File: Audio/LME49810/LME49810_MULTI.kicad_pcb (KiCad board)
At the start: 2 copper layers, 165.1 x 190.5 mm, 124 parts, among them Q1 NPN(TO-3P-BCE), Q2 PNP(TO-3P-BCE), Q3 NPN(TO-220-BCE), U1 LME49810

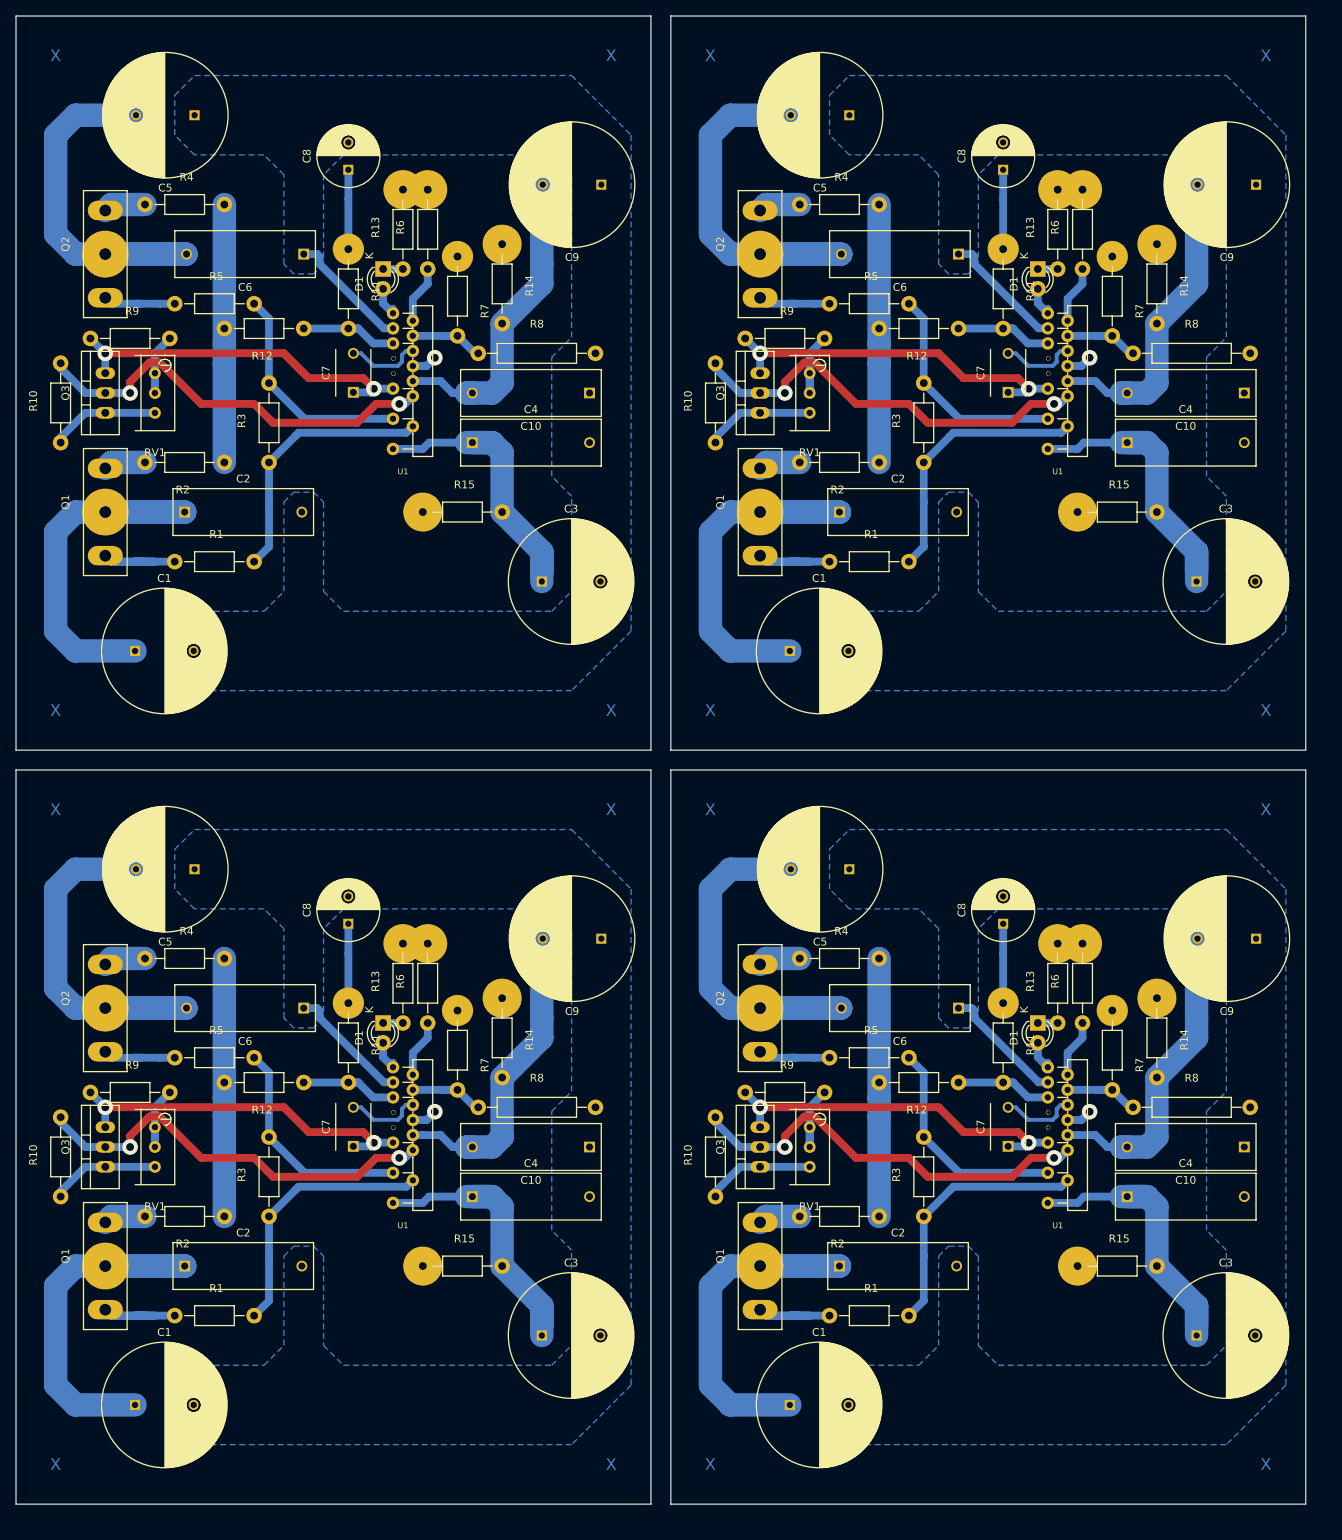
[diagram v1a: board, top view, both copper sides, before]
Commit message: Fixes
More fixes done
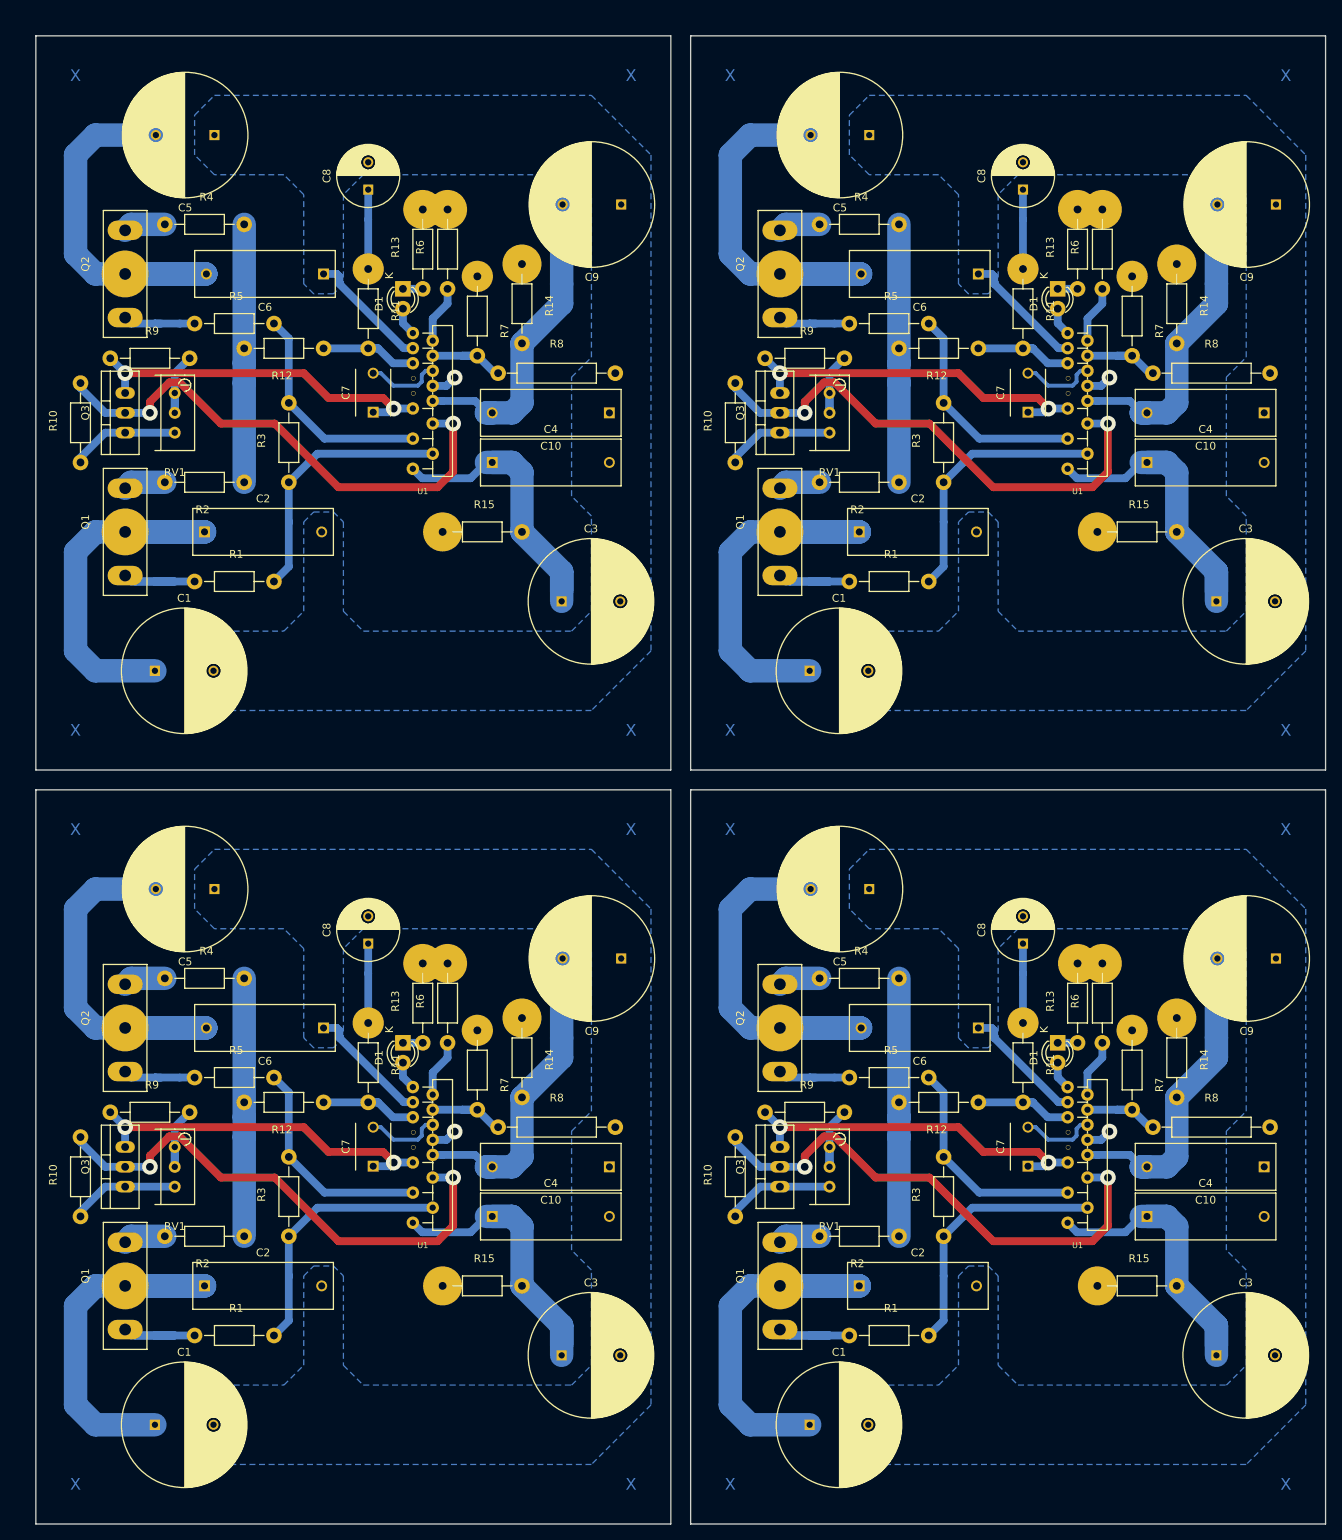
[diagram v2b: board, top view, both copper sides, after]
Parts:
- removed the C1 at (33.0, 99.1)
- removed the C1 at (116.8, 99.1)
- removed the C1 at (33.0, 195.6)
- removed the C1 at (116.8, 195.6)
- removed the C10 at (91.2, 66.0)
- removed the C10 at (175.0, 66.0)
- removed the C10 at (91.2, 162.6)
- removed the C10 at (175.0, 162.6)
- removed the C2 at (39.4, 81.3)
- removed the C2 at (123.2, 81.3)
- removed the C2 at (39.4, 177.8)
- removed the C2 at (123.2, 177.8)
- removed the C3 at (85.1, 90.2)
- removed the C3 at (168.9, 90.2)
- removed the C3 at (85.1, 186.7)
- removed the C3 at (168.9, 186.7)
- removed the C4 at (76.2, 72.4)
- removed the C4 at (160.0, 72.4)
- removed the C4 at (76.2, 168.9)
- removed the C4 at (160.0, 168.9)
- removed the C5 at (40.6, 30.5)
- removed the C5 at (124.5, 30.5)
- removed the C5 at (40.6, 127.0)
- removed the C5 at (124.5, 127.0)
- removed the C6 at (54.6, 48.3)
- removed the C6 at (138.4, 48.3)
- removed the C6 at (54.6, 144.8)
- removed the C6 at (138.4, 144.8)
- removed the C7 at (61.0, 66.0)
- removed the C7 at (144.8, 66.0)
- removed the C7 at (61.0, 162.5)
- removed the C7 at (144.8, 162.5)
- removed the C8 at (60.3, 37.5)
- removed the C8 at (144.1, 37.5)
- removed the C8 at (60.3, 134.0)
- removed the C8 at (144.1, 134.0)
- removed the C9 at (92.7, 39.4)
- removed the C9 at (176.5, 39.4)
- removed the C9 at (92.7, 135.9)
- removed the C9 at (176.5, 135.9)
- removed the D1 at (64.8, 50.2)
- removed the D1 at (148.6, 50.2)
- removed the D1 at (64.8, 146.7)
- removed the D1 at (148.6, 146.7)
- removed the Q1 at (29.2, 81.3)
- removed the Q1 at (113.0, 81.3)
- removed the Q1 at (29.2, 177.8)
- removed the Q1 at (113.0, 177.8)
- removed the Q2 at (29.2, 48.3)
- removed the Q2 at (113.0, 48.3)
- removed the Q2 at (29.2, 144.8)
- removed the Q2 at (113.0, 144.8)
- removed the Q3 at (29.2, 66.0)
- removed the Q3 at (113.0, 66.0)
- removed the Q3 at (29.2, 162.6)
- removed the Q3 at (113.0, 162.6)
- removed the R1 at (43.2, 87.6)
- removed the R1 at (127.0, 87.6)
- removed the R1 at (43.2, 184.2)
- removed the R1 at (127.0, 184.2)
- removed the R10 at (23.5, 67.3)
- removed the R10 at (107.3, 67.3)
- removed the R10 at (23.5, 163.8)
- removed the R10 at (107.3, 163.8)
- removed the R11 at (60.3, 52.7)
- removed the R11 at (144.1, 52.7)
- removed the R11 at (60.3, 149.2)
- removed the R11 at (144.1, 149.2)
- removed the R12 at (49.5, 57.8)
- removed the R12 at (133.3, 57.8)
- removed the R12 at (49.5, 154.3)
- removed the R12 at (133.3, 154.3)
- removed the R13 at (67.3, 45.1)
- removed the R13 at (151.1, 45.1)
- removed the R13 at (67.3, 141.6)
- removed the R13 at (151.1, 141.6)
- removed the R14 at (80.0, 52.1)
- removed the R14 at (163.8, 52.1)
- removed the R14 at (80.0, 148.6)
- removed the R14 at (163.8, 148.6)
- removed the R15 at (74.9, 81.3)
- removed the R15 at (158.8, 81.3)
- removed the R15 at (74.9, 177.8)
- removed the R15 at (158.8, 177.8)
- removed the R2 at (39.4, 74.9)
- removed the R2 at (123.2, 74.9)
- removed the R2 at (39.4, 171.4)
- removed the R2 at (123.2, 171.4)
- removed the R3 at (50.2, 69.8)
- removed the R3 at (134.0, 69.8)
- removed the R3 at (50.2, 166.4)
- removed the R3 at (134.0, 166.4)
- removed the R4 at (39.4, 41.9)
- removed the R4 at (123.2, 41.9)
- removed the R4 at (39.4, 138.4)
- removed the R4 at (123.2, 138.4)
- removed the R5 at (43.2, 54.6)
- removed the R5 at (127.0, 54.6)
- removed the R5 at (43.2, 151.1)
- removed the R5 at (127.0, 151.1)
- removed the R6 at (70.5, 45.1)
- removed the R6 at (154.3, 45.1)
- removed the R6 at (70.5, 141.6)
- removed the R6 at (154.3, 141.6)
- removed the R7 at (74.3, 53.6)
- removed the R7 at (158.1, 53.6)
- removed the R7 at (74.3, 150.2)
- removed the R7 at (158.1, 150.2)
- removed the R8 at (84.5, 61.0)
- removed the R8 at (168.3, 61.0)
- removed the R8 at (84.5, 157.5)
- removed the R8 at (168.3, 157.5)
- removed the R9 at (32.4, 59.1)
- removed the R9 at (116.2, 59.1)
- removed the R9 at (32.4, 155.6)
- removed the R9 at (116.2, 155.6)
- removed the RV1 at (35.6, 63.5)
- removed the RV1 at (119.4, 63.5)
- removed the RV1 at (35.6, 160.0)
- removed the RV1 at (119.4, 160.0)
- removed the U1 at (67.3, 64.5)
- removed the U1 at (151.1, 64.5)
- removed the U1 at (67.3, 161.0)
- removed the U1 at (151.1, 161.0)
- added C1: 820u,100V, Capacitors_ThroughHole:C_Radial_D16_L31.5_P7.5, F.Cu at (35.6, 101.6)
- added C1: 820u,100V, Capacitors_ThroughHole:C_Radial_D16_L31.5_P7.5, F.Cu at (119.4, 101.6)
- added C1: 820u,100V, Capacitors_ThroughHole:C_Radial_D16_L31.5_P7.5, F.Cu at (35.6, 198.1)
- added C1: 820u,100V, Capacitors_ThroughHole:C_Radial_D16_L31.5_P7.5, F.Cu at (119.4, 198.1)
- added C10: 0.1u, Capacitors_ThroughHole:C_Rect_L18_W6_H12_P15, F.Cu at (93.7, 68.6)
- added C10: 0.1u, Capacitors_ThroughHole:C_Rect_L18_W6_H12_P15, F.Cu at (177.6, 68.6)
- added C10: 0.1u, Capacitors_ThroughHole:C_Rect_L18_W6_H12_P15, F.Cu at (93.7, 165.1)
- added C10: 0.1u, Capacitors_ThroughHole:C_Rect_L18_W6_H12_P15, F.Cu at (177.6, 165.1)
- added C2: 0.1u, Capacitors_ThroughHole:C_Rect_L18_W6_H12_P15, F.Cu at (41.9, 83.8)
- added C2: 0.1u, Capacitors_ThroughHole:C_Rect_L18_W6_H12_P15, F.Cu at (125.7, 83.8)
- added C2: 0.1u, Capacitors_ThroughHole:C_Rect_L18_W6_H12_P15, F.Cu at (41.9, 180.3)
- added C2: 0.1u, Capacitors_ThroughHole:C_Rect_L18_W6_H12_P15, F.Cu at (125.7, 180.3)
- added C3: 820u,100V, Capacitors_ThroughHole:C_Radial_D16_L31.5_P7.5, F.Cu at (87.6, 92.7)
- added C3: 820u,100V, Capacitors_ThroughHole:C_Radial_D16_L31.5_P7.5, F.Cu at (171.4, 92.7)
- added C3: 820u,100V, Capacitors_ThroughHole:C_Radial_D16_L31.5_P7.5, F.Cu at (87.6, 189.2)
- added C3: 820u,100V, Capacitors_ThroughHole:C_Radial_D16_L31.5_P7.5, F.Cu at (171.4, 189.2)
- added C4: 0.1u, Capacitors_ThroughHole:C_Rect_L18_W6_H12_P15, F.Cu at (78.7, 74.9)
- added C4: 0.1u, Capacitors_ThroughHole:C_Rect_L18_W6_H12_P15, F.Cu at (162.6, 74.9)
- added C4: 0.1u, Capacitors_ThroughHole:C_Rect_L18_W6_H12_P15, F.Cu at (78.7, 171.4)
- added C4: 0.1u, Capacitors_ThroughHole:C_Rect_L18_W6_H12_P15, F.Cu at (162.6, 171.4)
- added C5: 820u,100V, Capacitors_ThroughHole:C_Radial_D16_L31.5_P7.5, F.Cu at (43.2, 33.0)
- added C5: 820u,100V, Capacitors_ThroughHole:C_Radial_D16_L31.5_P7.5, F.Cu at (127.0, 33.0)
- added C5: 820u,100V, Capacitors_ThroughHole:C_Radial_D16_L31.5_P7.5, F.Cu at (43.2, 129.5)
- added C5: 820u,100V, Capacitors_ThroughHole:C_Radial_D16_L31.5_P7.5, F.Cu at (127.0, 129.5)
- added C6: 0.1u, Capacitors_ThroughHole:C_Rect_L18_W6_H12_P15, F.Cu at (57.1, 50.8)
- added C6: 0.1u, Capacitors_ThroughHole:C_Rect_L18_W6_H12_P15, F.Cu at (141.0, 50.8)
- added C6: 0.1u, Capacitors_ThroughHole:C_Rect_L18_W6_H12_P15, F.Cu at (57.1, 147.3)
- added C6: 0.1u, Capacitors_ThroughHole:C_Rect_L18_W6_H12_P15, F.Cu at (141.0, 147.3)
- added C7: 10p, Capacitors_ThroughHole:C_Disc_D6_P5, F.Cu at (63.5, 68.5)
- added C7: 10p, Capacitors_ThroughHole:C_Disc_D6_P5, F.Cu at (147.3, 68.5)
- added C7: 10p, Capacitors_ThroughHole:C_Disc_D6_P5, F.Cu at (63.5, 165.0)
- added C7: 10p, Capacitors_ThroughHole:C_Disc_D6_P5, F.Cu at (147.3, 165.0)
- added C8: 220u, Capacitors_ThroughHole:C_Radial_D8_L11.5_P3.5, F.Cu at (62.9, 40.0)
- added C8: 220u, Capacitors_ThroughHole:C_Radial_D8_L11.5_P3.5, F.Cu at (146.7, 40.0)
- added C8: 220u, Capacitors_ThroughHole:C_Radial_D8_L11.5_P3.5, F.Cu at (62.9, 136.5)
- added C8: 220u, Capacitors_ThroughHole:C_Radial_D8_L11.5_P3.5, F.Cu at (146.7, 136.5)
- added C9: 820u,100V, Capacitors_ThroughHole:C_Radial_D16_L31.5_P7.5, F.Cu at (95.2, 41.9)
- added C9: 820u,100V, Capacitors_ThroughHole:C_Radial_D16_L31.5_P7.5, F.Cu at (179.1, 41.9)
- added C9: 820u,100V, Capacitors_ThroughHole:C_Radial_D16_L31.5_P7.5, F.Cu at (95.2, 138.4)
- added C9: 820u,100V, Capacitors_ThroughHole:C_Radial_D16_L31.5_P7.5, F.Cu at (179.1, 138.4)
- added D1: LED, LEDs:LED-3MM, F.Cu at (67.3, 52.7)
- added D1: LED, LEDs:LED-3MM, F.Cu at (151.1, 52.7)
- added D1: LED, LEDs:LED-3MM, F.Cu at (67.3, 149.2)
- added D1: LED, LEDs:LED-3MM, F.Cu at (151.1, 149.2)
- added Q1: NPN(TO-3P-BCE), Transistors_TO-247:TO-247_Vertical_Neutral123, F.Cu at (31.8, 83.8)
- added Q1: NPN(TO-3P-BCE), Transistors_TO-247:TO-247_Vertical_Neutral123, F.Cu at (115.6, 83.8)
- added Q1: NPN(TO-3P-BCE), Transistors_TO-247:TO-247_Vertical_Neutral123, F.Cu at (31.8, 180.3)
- added Q1: NPN(TO-3P-BCE), Transistors_TO-247:TO-247_Vertical_Neutral123, F.Cu at (115.6, 180.3)
- added Q2: PNP(TO-3P-BCE), Transistors_TO-247:TO-247_Vertical_Neutral123, F.Cu at (31.8, 50.8)
- added Q2: PNP(TO-3P-BCE), Transistors_TO-247:TO-247_Vertical_Neutral123, F.Cu at (115.6, 50.8)
- added Q2: PNP(TO-3P-BCE), Transistors_TO-247:TO-247_Vertical_Neutral123, F.Cu at (31.8, 147.3)
- added Q2: PNP(TO-3P-BCE), Transistors_TO-247:TO-247_Vertical_Neutral123, F.Cu at (115.6, 147.3)
- added Q3: NPN(TO-220-BCE), Transistors_TO-220:TO-220_Neutral123_Vertical, F.Cu at (31.8, 68.6)
- added Q3: NPN(TO-220-BCE), Transistors_TO-220:TO-220_Neutral123_Vertical, F.Cu at (115.6, 68.6)
- added Q3: NPN(TO-220-BCE), Transistors_TO-220:TO-220_Neutral123_Vertical, F.Cu at (31.8, 165.1)
- added Q3: NPN(TO-220-BCE), Transistors_TO-220:TO-220_Neutral123_Vertical, F.Cu at (115.6, 165.1)
- added R1: 100, Resistors_ThroughHole:Resistor_Horizontal_RM10mm, F.Cu at (45.7, 90.2)
- added R1: 100, Resistors_ThroughHole:Resistor_Horizontal_RM10mm, F.Cu at (129.5, 90.2)
- added R1: 100, Resistors_ThroughHole:Resistor_Horizontal_RM10mm, F.Cu at (45.7, 186.7)
- added R1: 100, Resistors_ThroughHole:Resistor_Horizontal_RM10mm, F.Cu at (129.5, 186.7)
- added R10: 1.2k, Resistors_ThroughHole:Resistor_Horizontal_RM10mm, F.Cu at (26.0, 69.8)
- added R10: 1.2k, Resistors_ThroughHole:Resistor_Horizontal_RM10mm, F.Cu at (109.9, 69.8)
- added R10: 1.2k, Resistors_ThroughHole:Resistor_Horizontal_RM10mm, F.Cu at (26.0, 166.4)
- added R10: 1.2k, Resistors_ThroughHole:Resistor_Horizontal_RM10mm, F.Cu at (109.9, 166.4)
- added R11: 240, Resistors_ThroughHole:Resistor_Horizontal_RM10mm, F.Cu at (62.9, 55.2)
- added R11: 240, Resistors_ThroughHole:Resistor_Horizontal_RM10mm, F.Cu at (146.7, 55.2)
- added R11: 240, Resistors_ThroughHole:Resistor_Horizontal_RM10mm, F.Cu at (62.9, 151.8)
- added R11: 240, Resistors_ThroughHole:Resistor_Horizontal_RM10mm, F.Cu at (146.7, 151.8)
- added R12: 6.8k, Resistors_ThroughHole:Resistor_Horizontal_RM10mm, F.Cu at (52.1, 60.3)
- added R12: 6.8k, Resistors_ThroughHole:Resistor_Horizontal_RM10mm, F.Cu at (135.9, 60.3)
- added R12: 6.8k, Resistors_ThroughHole:Resistor_Horizontal_RM10mm, F.Cu at (52.1, 156.8)
- added R12: 6.8k, Resistors_ThroughHole:Resistor_Horizontal_RM10mm, F.Cu at (135.9, 156.8)
- added R13: 470, Resistors_ThroughHole:Resistor_Horizontal_RM10mm, F.Cu at (69.8, 47.6)
- added R13: 470, Resistors_ThroughHole:Resistor_Horizontal_RM10mm, F.Cu at (153.7, 47.6)
- added R13: 470, Resistors_ThroughHole:Resistor_Horizontal_RM10mm, F.Cu at (69.8, 144.1)
- added R13: 470, Resistors_ThroughHole:Resistor_Horizontal_RM10mm, F.Cu at (153.7, 144.1)
- added R14: 10, Resistors_ThroughHole:Resistor_Horizontal_RM10mm, F.Cu at (82.5, 54.6)
- added R14: 10, Resistors_ThroughHole:Resistor_Horizontal_RM10mm, F.Cu at (166.4, 54.6)
- added R14: 10, Resistors_ThroughHole:Resistor_Horizontal_RM10mm, F.Cu at (82.5, 151.1)
- added R14: 10, Resistors_ThroughHole:Resistor_Horizontal_RM10mm, F.Cu at (166.4, 151.1)
- added R15: 10, Resistors_ThroughHole:Resistor_Horizontal_RM10mm, F.Cu at (77.5, 83.8)
- added R15: 10, Resistors_ThroughHole:Resistor_Horizontal_RM10mm, F.Cu at (161.3, 83.8)
- added R15: 10, Resistors_ThroughHole:Resistor_Horizontal_RM10mm, F.Cu at (77.5, 180.3)
- added R15: 10, Resistors_ThroughHole:Resistor_Horizontal_RM10mm, F.Cu at (161.3, 180.3)
- added R2: 0.22, Resistors_ThroughHole:Resistor_Horizontal_RM10mm, F.Cu at (41.9, 77.5)
- added R2: 0.22, Resistors_ThroughHole:Resistor_Horizontal_RM10mm, F.Cu at (125.7, 77.5)
- added R2: 0.22, Resistors_ThroughHole:Resistor_Horizontal_RM10mm, F.Cu at (41.9, 174.0)
- added R2: 0.22, Resistors_ThroughHole:Resistor_Horizontal_RM10mm, F.Cu at (125.7, 174.0)
- added R3: 2.2k, Resistors_ThroughHole:Resistor_Horizontal_RM10mm, F.Cu at (52.7, 72.4)
- added R3: 2.2k, Resistors_ThroughHole:Resistor_Horizontal_RM10mm, F.Cu at (136.5, 72.4)
- added R3: 2.2k, Resistors_ThroughHole:Resistor_Horizontal_RM10mm, F.Cu at (52.7, 168.9)
- added R3: 2.2k, Resistors_ThroughHole:Resistor_Horizontal_RM10mm, F.Cu at (136.5, 168.9)
- added R4: 0.22, Resistors_ThroughHole:Resistor_Horizontal_RM10mm, F.Cu at (41.9, 44.5)
- added R4: 0.22, Resistors_ThroughHole:Resistor_Horizontal_RM10mm, F.Cu at (125.7, 44.5)
- added R4: 0.22, Resistors_ThroughHole:Resistor_Horizontal_RM10mm, F.Cu at (41.9, 141.0)
- added R4: 0.22, Resistors_ThroughHole:Resistor_Horizontal_RM10mm, F.Cu at (125.7, 141.0)
- added R5: 100, Resistors_ThroughHole:Resistor_Horizontal_RM10mm, F.Cu at (45.7, 57.1)
- added R5: 100, Resistors_ThroughHole:Resistor_Horizontal_RM10mm, F.Cu at (129.5, 57.1)
- added R5: 100, Resistors_ThroughHole:Resistor_Horizontal_RM10mm, F.Cu at (45.7, 153.7)
- added R5: 100, Resistors_ThroughHole:Resistor_Horizontal_RM10mm, F.Cu at (129.5, 153.7)
- added R6: 33k, Resistors_ThroughHole:Resistor_Horizontal_RM10mm, F.Cu at (73.0, 47.6)
- added R6: 33k, Resistors_ThroughHole:Resistor_Horizontal_RM10mm, F.Cu at (156.8, 47.6)
- added R6: 33k, Resistors_ThroughHole:Resistor_Horizontal_RM10mm, F.Cu at (73.0, 144.1)
- added R6: 33k, Resistors_ThroughHole:Resistor_Horizontal_RM10mm, F.Cu at (156.8, 144.1)
- added R7: 240, Resistors_ThroughHole:Resistor_Horizontal_RM10mm, F.Cu at (76.8, 56.2)
- added R7: 240, Resistors_ThroughHole:Resistor_Horizontal_RM10mm, F.Cu at (160.7, 56.2)
- added R7: 240, Resistors_ThroughHole:Resistor_Horizontal_RM10mm, F.Cu at (76.8, 152.7)
- added R7: 240, Resistors_ThroughHole:Resistor_Horizontal_RM10mm, F.Cu at (160.7, 152.7)
- added R8: 6.8k, Resistors_ThroughHole:Resistor_Horizontal_RM15mm, F.Cu at (87.0, 63.5)
- added R8: 6.8k, Resistors_ThroughHole:Resistor_Horizontal_RM15mm, F.Cu at (170.8, 63.5)
- added R8: 6.8k, Resistors_ThroughHole:Resistor_Horizontal_RM15mm, F.Cu at (87.0, 160.0)
- added R8: 6.8k, Resistors_ThroughHole:Resistor_Horizontal_RM15mm, F.Cu at (170.8, 160.0)
- added R9: 360, Resistors_ThroughHole:Resistor_Horizontal_RM10mm, F.Cu at (34.9, 61.6)
- added R9: 360, Resistors_ThroughHole:Resistor_Horizontal_RM10mm, F.Cu at (118.7, 61.6)
- added R9: 360, Resistors_ThroughHole:Resistor_Horizontal_RM10mm, F.Cu at (34.9, 158.1)
- added R9: 360, Resistors_ThroughHole:Resistor_Horizontal_RM10mm, F.Cu at (118.7, 158.1)
- added RV1: 200, Potentiometers:Potentiometer_Bourns_3296W_3-8Zoll_Inline_ScrewUp, F.Cu at (38.1, 66.0)
- added RV1: 200, Potentiometers:Potentiometer_Bourns_3296W_3-8Zoll_Inline_ScrewUp, F.Cu at (121.9, 66.0)
- added RV1: 200, Potentiometers:Potentiometer_Bourns_3296W_3-8Zoll_Inline_ScrewUp, F.Cu at (38.1, 162.6)
- added RV1: 200, Potentiometers:Potentiometer_Bourns_3296W_3-8Zoll_Inline_ScrewUp, F.Cu at (121.9, 162.6)
- added U1: LME49810, LME49810:LME49810, F.Cu at (69.8, 67.1)
- added U1: LME49810, LME49810:LME49810, F.Cu at (153.7, 67.1)
- added U1: LME49810, LME49810:LME49810, F.Cu at (69.8, 163.6)
- added U1: LME49810, LME49810:LME49810, F.Cu at (153.7, 163.6)
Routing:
- net CLH: track 216.3 -> 269.1 mm
- net Net-(C3-Pad1): track 154.1 -> 158.2 mm
- net Net-(D1-Pad2): track 16.6 -> 14.6 mm
- net SourceLH: track 135.3 -> 133.7 mm
